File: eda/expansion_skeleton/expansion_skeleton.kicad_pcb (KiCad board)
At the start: 2 copper layers, 217.2 x 104.1 mm, 14 parts, among them J2 Expansion

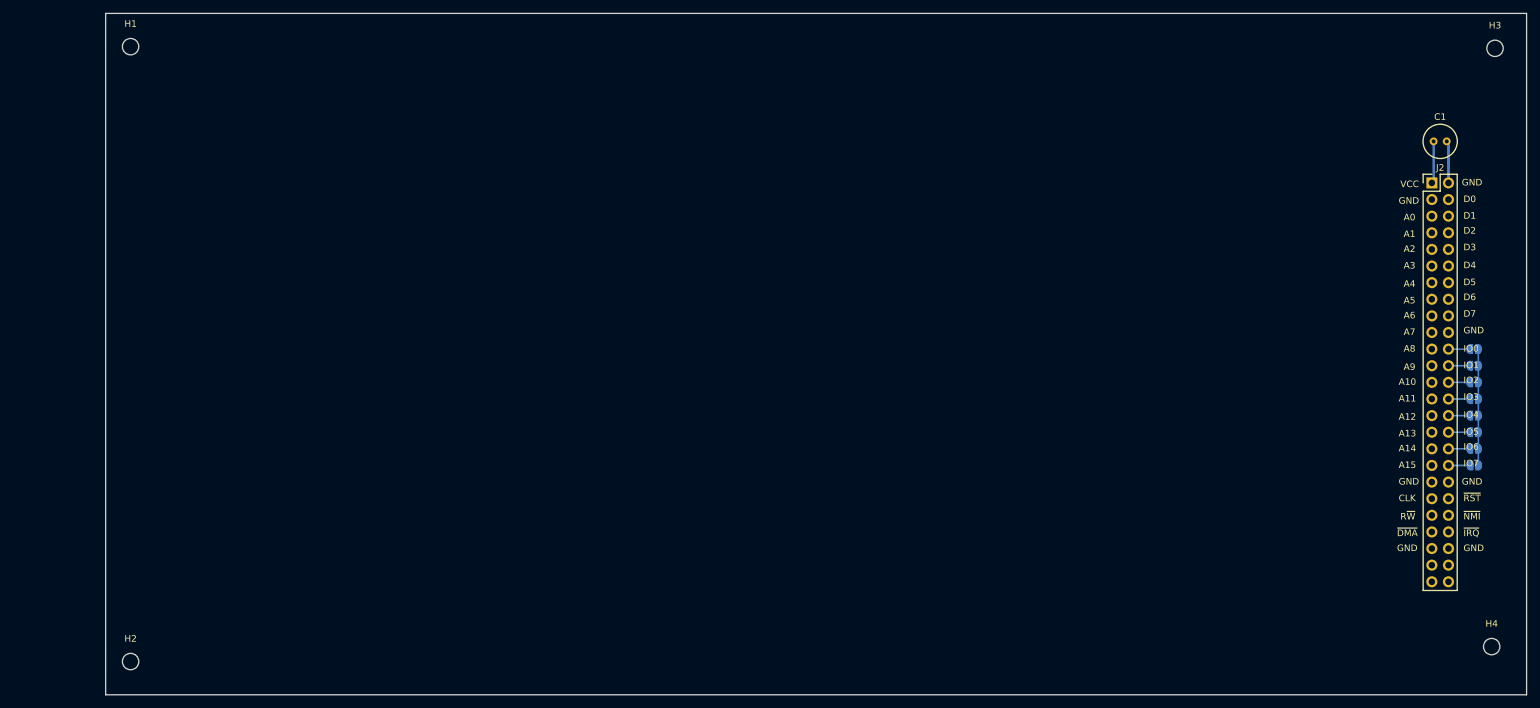
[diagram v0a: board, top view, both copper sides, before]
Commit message: Branch of uart to v1
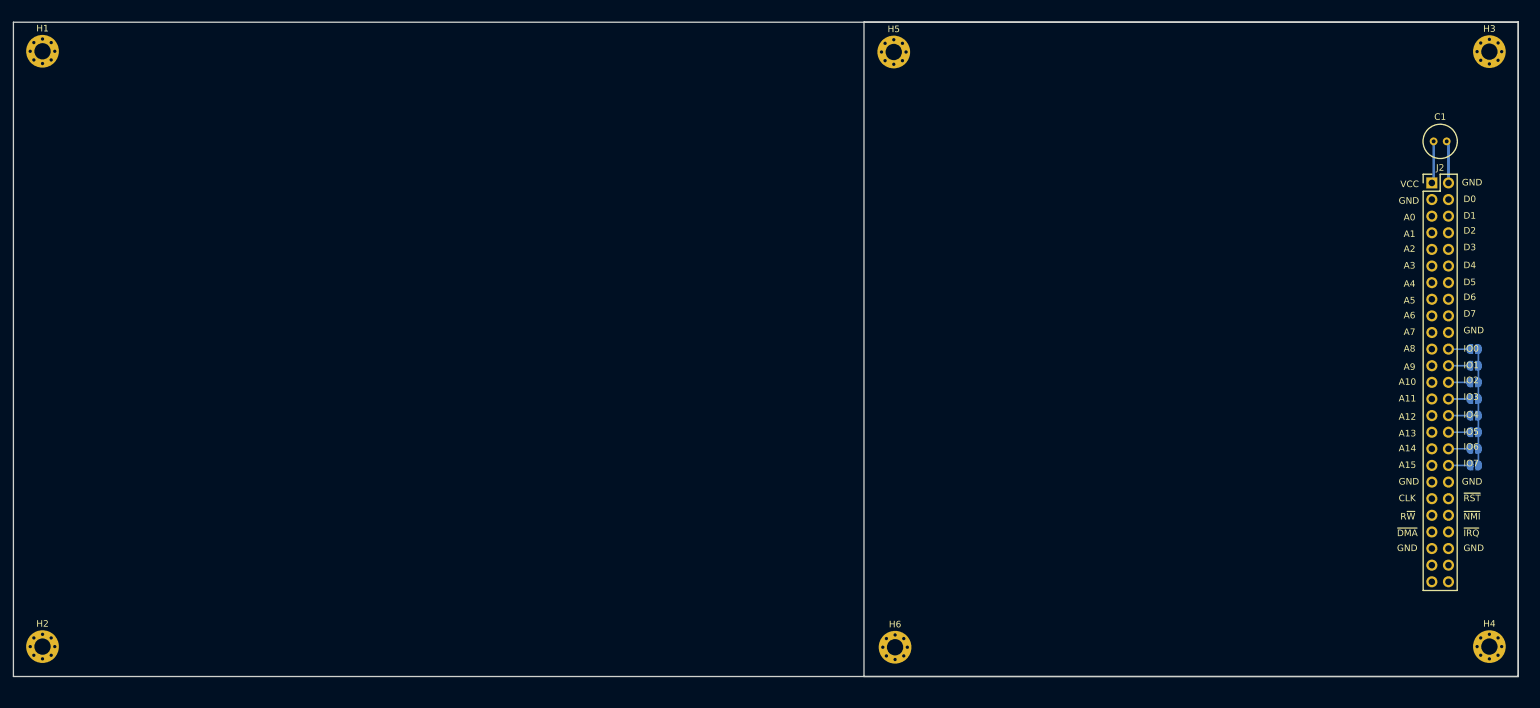
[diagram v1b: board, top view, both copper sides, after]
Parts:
- added H5: MountingHole_Pad, MountingHole:MountingHole_2.5mm_Pad_Via, F.Cu at (150.2, 26.0)
- added H6: MountingHole_Pad, MountingHole:MountingHole_2.5mm_Pad_Via, F.Cu at (150.4, 116.9)
- H1, H2, H3, H4: value Standoffs -> MountingHole_Pad; footprint MountingHole:MountingHole_2.5mm -> MountingHole:MountingHole_2.5mm_Pad_Via
- J2: value Expansion -> Conn_02x25_Odd_Even
- moved H2 13.7 mm to (20.1, 116.8)
- moved H1 13.5 mm to (20.1, 25.9)
- moved H3 1.00 mm to (241.2, 25.9)
- moved H4 0.35 mm to (241.2, 116.8)
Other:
- board size 217.2 x 104.1 mm -> 230 x 100 mm
